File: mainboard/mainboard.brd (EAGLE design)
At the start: 158.8 x 159.4 mm, 60 parts, among them T1 NPN_BC817,215, T2 NPN_BC817,215, T3 NPN_BC817,215

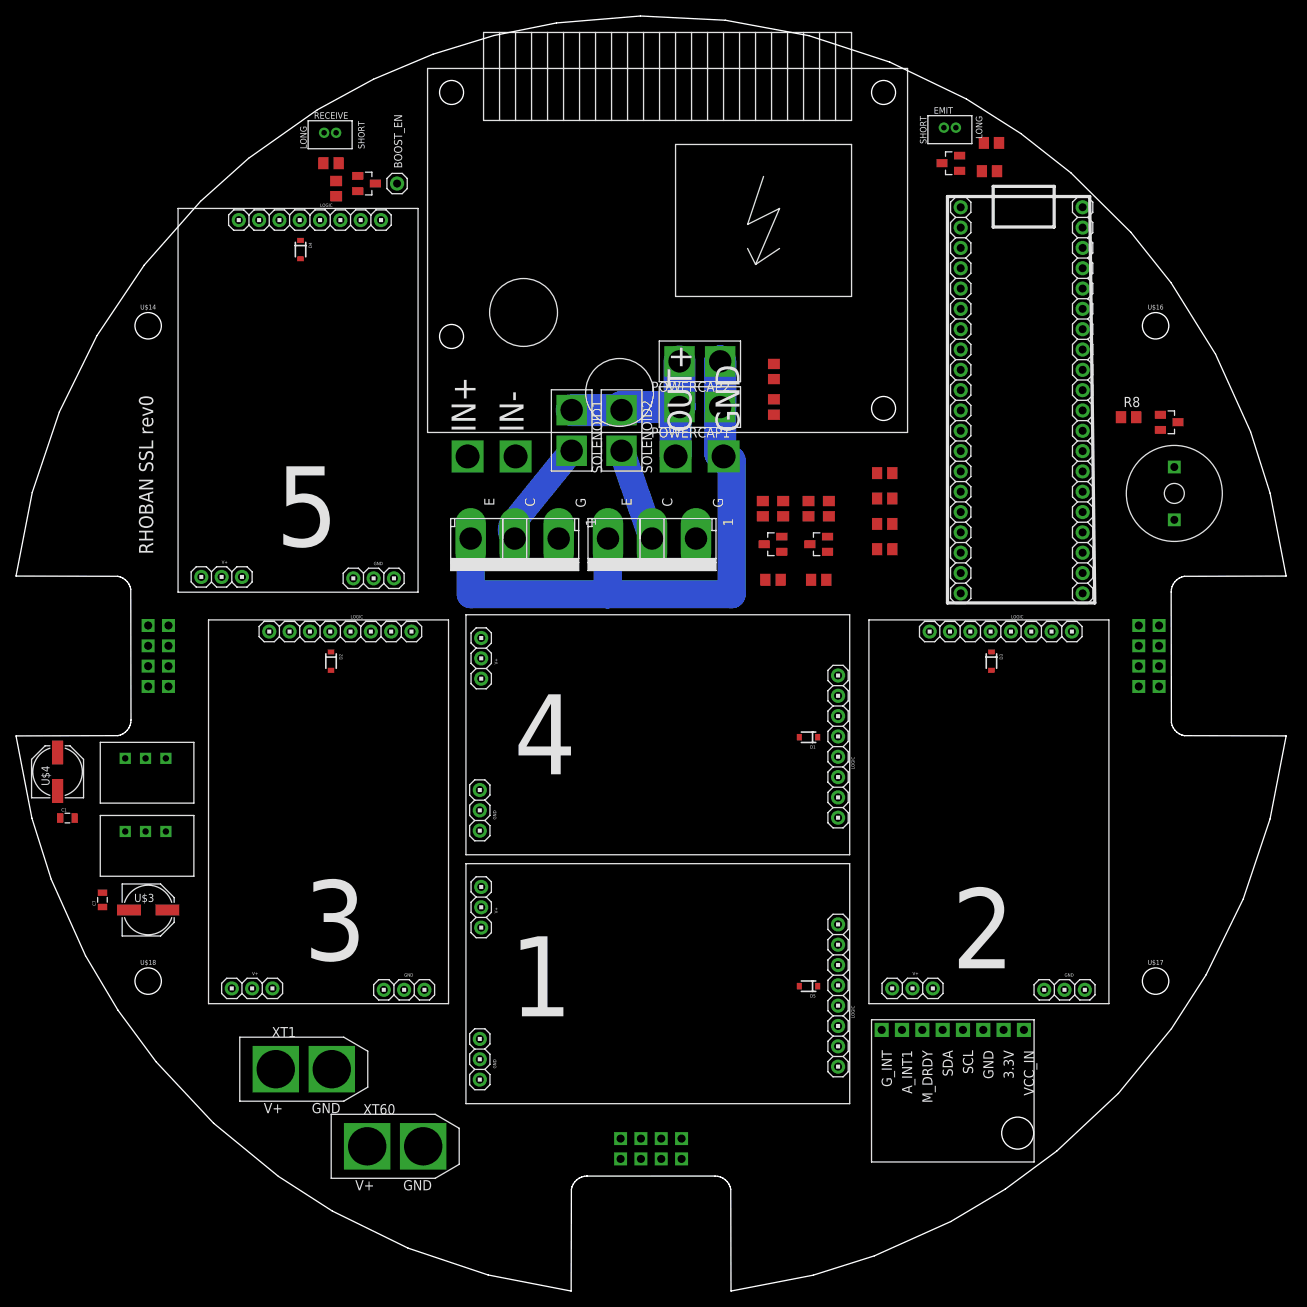
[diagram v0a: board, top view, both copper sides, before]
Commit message: Mainboard rev1 wip
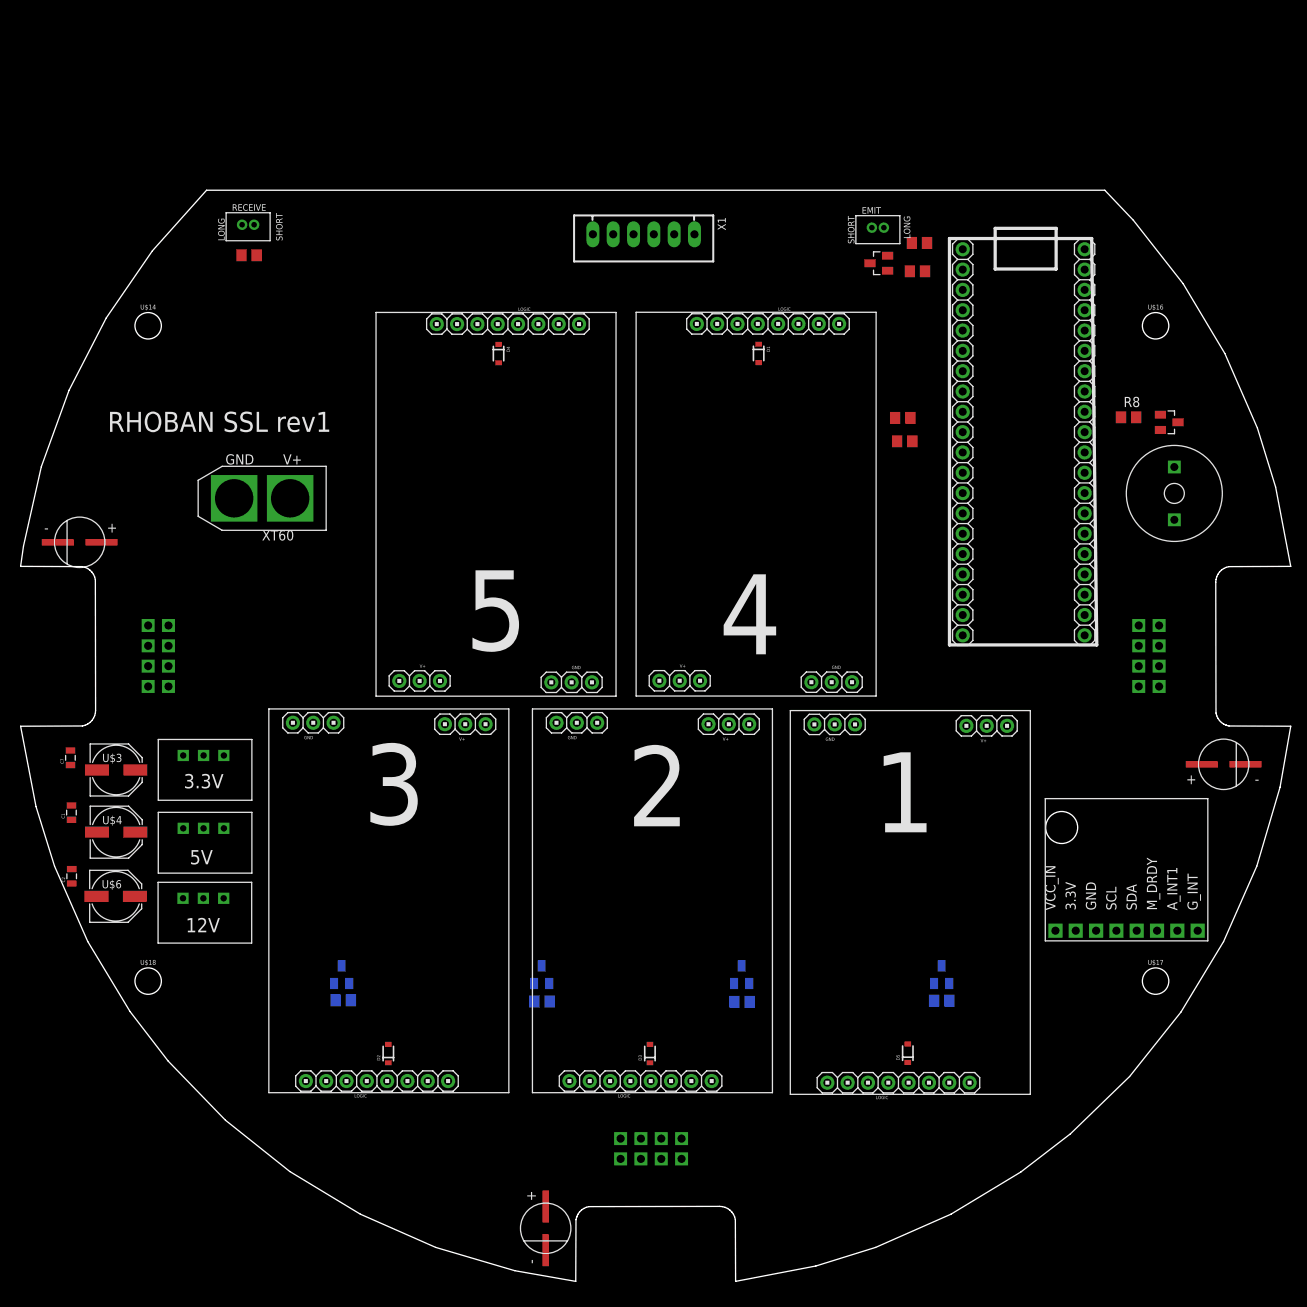
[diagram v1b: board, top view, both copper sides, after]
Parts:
- removed BOOST_EN: CONNEC_1X01, rhoban:CONNEC_1X01
- removed POWERCAP1, POWERCAP2, SOLENOID1, SOLENOID2: CONNEC_1X02BIG, rhoban:CONNEC_1X02_BIG
- removed R31, R9: 1K, rhoban:R0805
- removed R32, R33, R36: 3K, rhoban:R0805
- removed R34: 2M, rhoban:R0805
- removed R35: 10K, rhoban:R0805
- removed T1, T3, U$15: NPN_BC817,215, rhoban:SOT-23
- removed XT1: CONNEC_ALIM, rhoban:XT60
- added C2: 1uF, SparkFun-Passives:0805@1
- added REG3.3V1: REG_5V, rhoban:TRACOPOWER
- added U$10: DRV5023FAEDBZRQ1, rhoban:SOT-23
- added U$6: 47uF, rhoban:PANASONIC_D
- added U$7, U$8, U$9: (no value), rhoban:PANASONIC_D8
- added X1: JST-XH-06-PIN-LONG-PAD, Rembrandt Electronics - JST XH Connectors v1-0:JST-XH-06-PACKAGE-LONG-PAD
- R1: value 1K -> 10K
- R2, R3: value 3K -> 10K
- U$1, U$11: value TO-247A -> DRV5023FAEDBZRQ1; device to-247_n-channel_igbt:TO-247 -> rhoban:SOT-23
- U$5: value BOOSTER -> DRV5023FAEDBZRQ1; device rhoban:BOOSTER_390V -> rhoban:SOT-23
- moved R7 94.5 mm to (-35.3, -40.5), flipped to the bottom
- moved DRIVER4 90.6 mm to (-11.6, -50.1), turned to 0 degrees
- moved XT60 89.0 mm to (-37.4, 26.2), turned to 180 degrees
- moved U$5 78.3 mm to (14.5, -37.3), flipped to the bottom
- moved U$1 76.3 mm to (39.5, -37.3), flipped to the bottom, turned to 0 degrees
- moved U$11 66.9 mm to (-35.5, -37.3), flipped to the bottom, turned to 0 degrees
- moved DRIVER2 66.0 mm to (31.2, 43.5), turned to 180 degrees
- moved D3 65.0 mm to (3.03, -47.2), turned to 90 degrees
- moved R1 64.6 mm to (39.5, -40.5), flipped to the bottom, turned to 180 degrees
- moved R2 61.7 mm to (14.6, -40.7), flipped to the bottom, turned to 180 degrees
- moved R3 60.1 mm to (-10.4, -40.6), flipped to the bottom, turned to 180 degrees
- moved DRIVER3 59.5 mm to (-44.5, -50.1), turned to 0 degrees
- moved D2 49.6 mm to (-29.7, -47.2), turned to 90 degrees
- moved D1 48.4 mm to (16.6, 40.4), turned to 270 degrees
- moved U$2 41.4 mm to (71.5, -31.8), turned to 90 degrees
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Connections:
- net BAT2 renamed BAT
- removed net BAT1: MAPLE.X8, R7.1, R9.2
- removed net N$1: R1.2, T1.1
- removed net N$17: R31.2, T3.1
- removed net N$2: SOLENOID1.P$2, U$1.P$2
- removed net N$35: R33.1, T3.3, U$11.P$1
- removed net N$36: SOLENOID2.P$2, U$11.P$2
- removed net N$37: BOOST_EN.1, U$15.3
- removed net N$38: R36.1, U$15.1
- removed net N$4: R3.1, T1.3, U$1.P$1
- removed net VBOOST: POWERCAP1.P$2, POWERCAP2.P$2, R34.2, SOLENOID1.P$1, SOLENOID2.P$1, U$5.OUT+
- removed net VMID: D1.2, D2.2, D3.2, D4.2, D5.2, R7.2, XT1.GND, XT60.V+
- new net 12V: C2.2, D1.2, D2.2, D3.2, D4.2, D5.2, REG3.3V1.P$3, U$6.+
- new net HALL1: MAPLE.X14, R1.1, U$1.2
- new net HALL2: MAPLE.X8, R2.1, U$5.2
- new net HALL3: MAPLE.X2, R3.1, U$10.2
- new net HALL4: MAPLE.X31, R7.1, U$11.2
- net 3.3: now also R1.2, R3.2, R7.2, U$1.1, U$10.1, U$11.1, U$5.1, U$7.+, U$8.+, U$9.+; no longer R32.2
- net BOOST_EN: now also X1.3; no longer R36.2
- net CAP: now also X1.6; no longer R34.1, R35.2
- net GND: now also C2.1, REG3.3V1.P$2, U$1.3, U$10.3, U$11.3, U$5.3, U$6.-, U$7.-, U$8.-, U$9.-, X1.1; no longer POWERCAP1.P$1, POWERCAP2.P$1, R35.1, R9.1, T1.2, T3.2, U$1.P$3, U$11.P$3, U$15.2, U$5.IN-, U$5.OUT-
- net KICK1: now also X1.4; no longer R1.1, R2.1
- net KICK2: now also X1.5; no longer R31.1, R32.1
- net VIN: now also REG3.3V1.P$1, X1.2, XT60.V+; no longer R3.2, R33.2, U$5.VIN, XT1.V+
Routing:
- net GND: track 89.1 -> 0.00 mm
- net VBOOST: track 26.0 -> 0.00 mm
- net N$2: track 13.5 -> 0.00 mm
- net N$36: track 11.6 -> 0.00 mm
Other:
- board size 158.8 x 159.4 mm -> 158.8 x 136.4 mm
- board text added: "12V"
- board text added: "3.3V"
- board text added: "5V"
- board text added: "RHOBAN SSL rev1"
- board text removed: "BOOST_EN"
- board text removed: "REV0"
- board text removed: "RHOBAN SSL MAINBOARD"
- board text removed: "RHOBAN SSL rev0"
